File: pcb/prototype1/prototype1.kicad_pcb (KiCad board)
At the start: 2 copper layers, 73.4 x 73.4 mm, 87 parts, among them P5 USB_B, SW2 Button, SW3 Button, SW4 Button, SW5 Button, U1 STM32F401, U10 AT25_EEPROM, U11 LD1117S33CTR, U2 MP34DT01-M, U3 L3GD20HTR, U4 LIS331HH, U5 LIS331HH, U6 TPS61021, U7 TLC5926, U8 TLC5926, U9 TLC5926

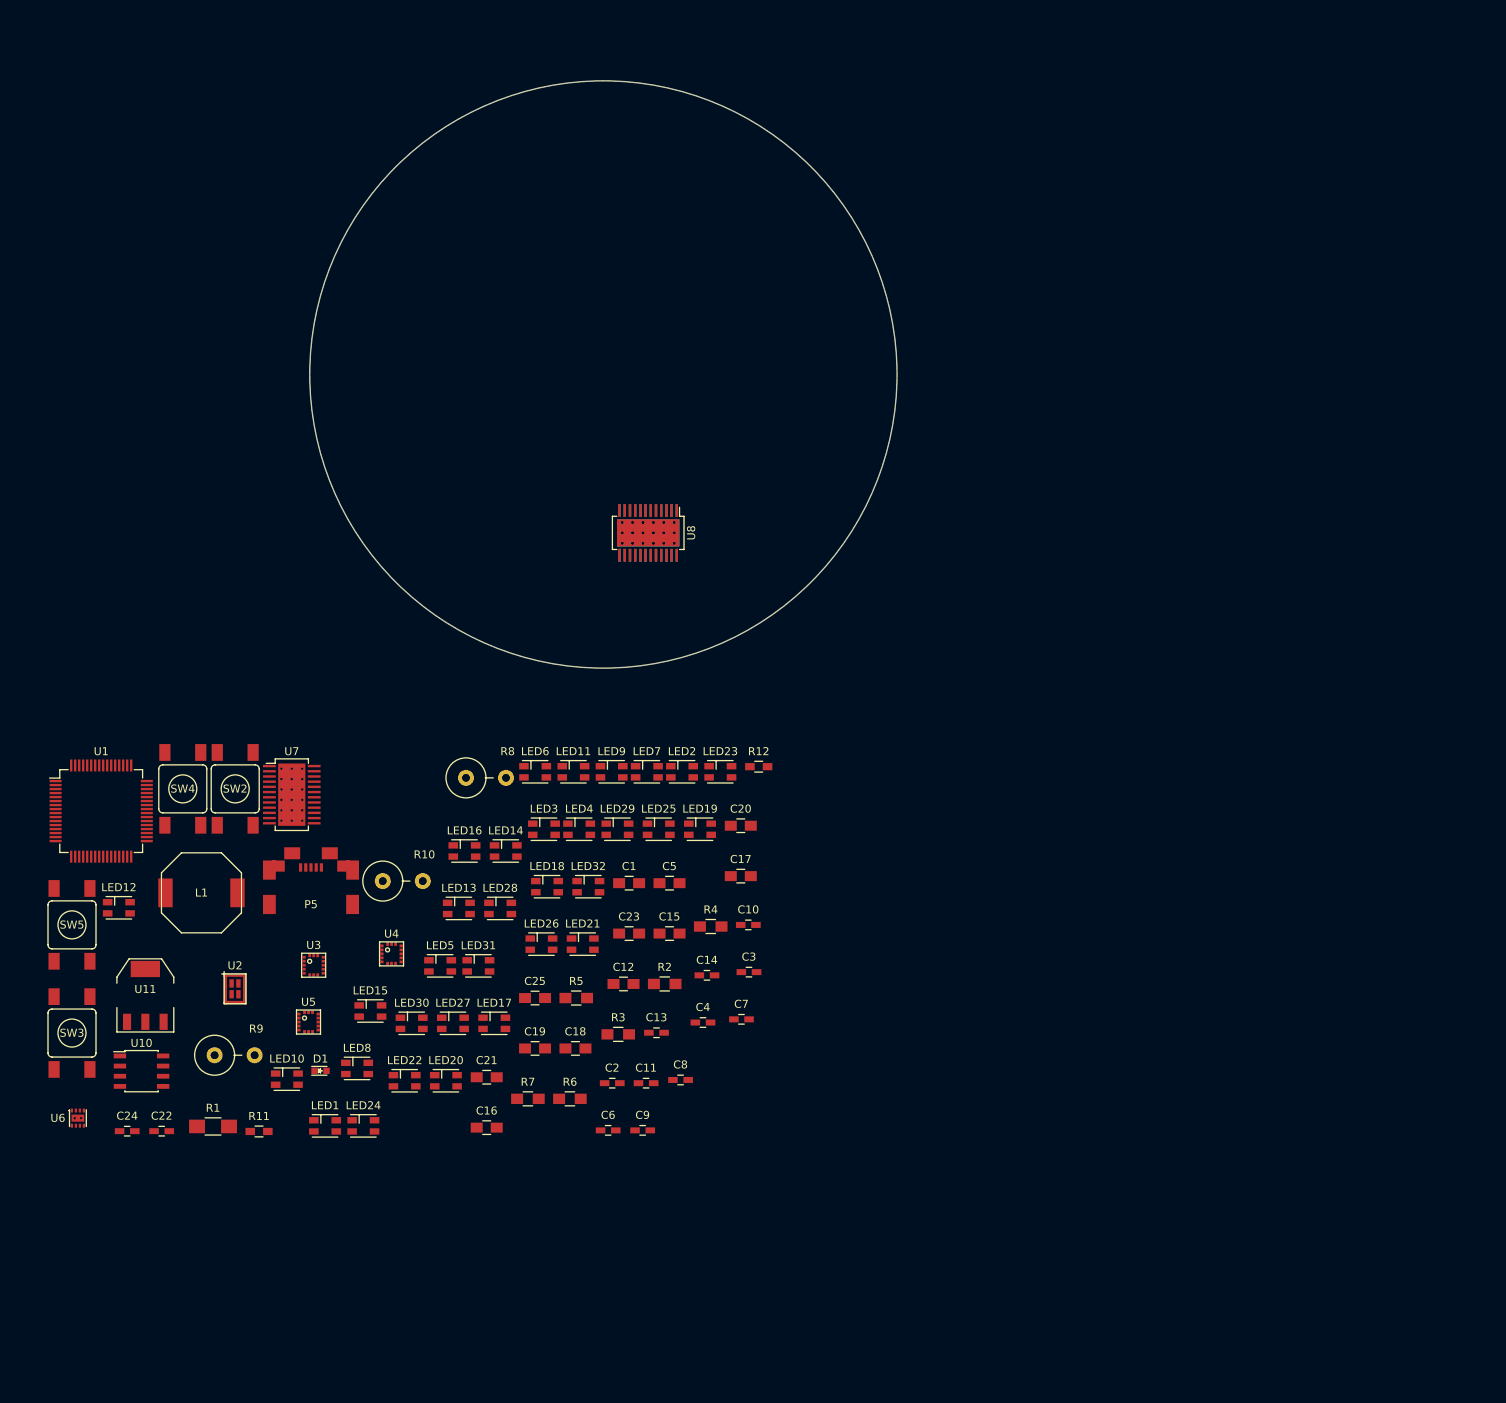
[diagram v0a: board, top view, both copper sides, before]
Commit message: Working on schematic
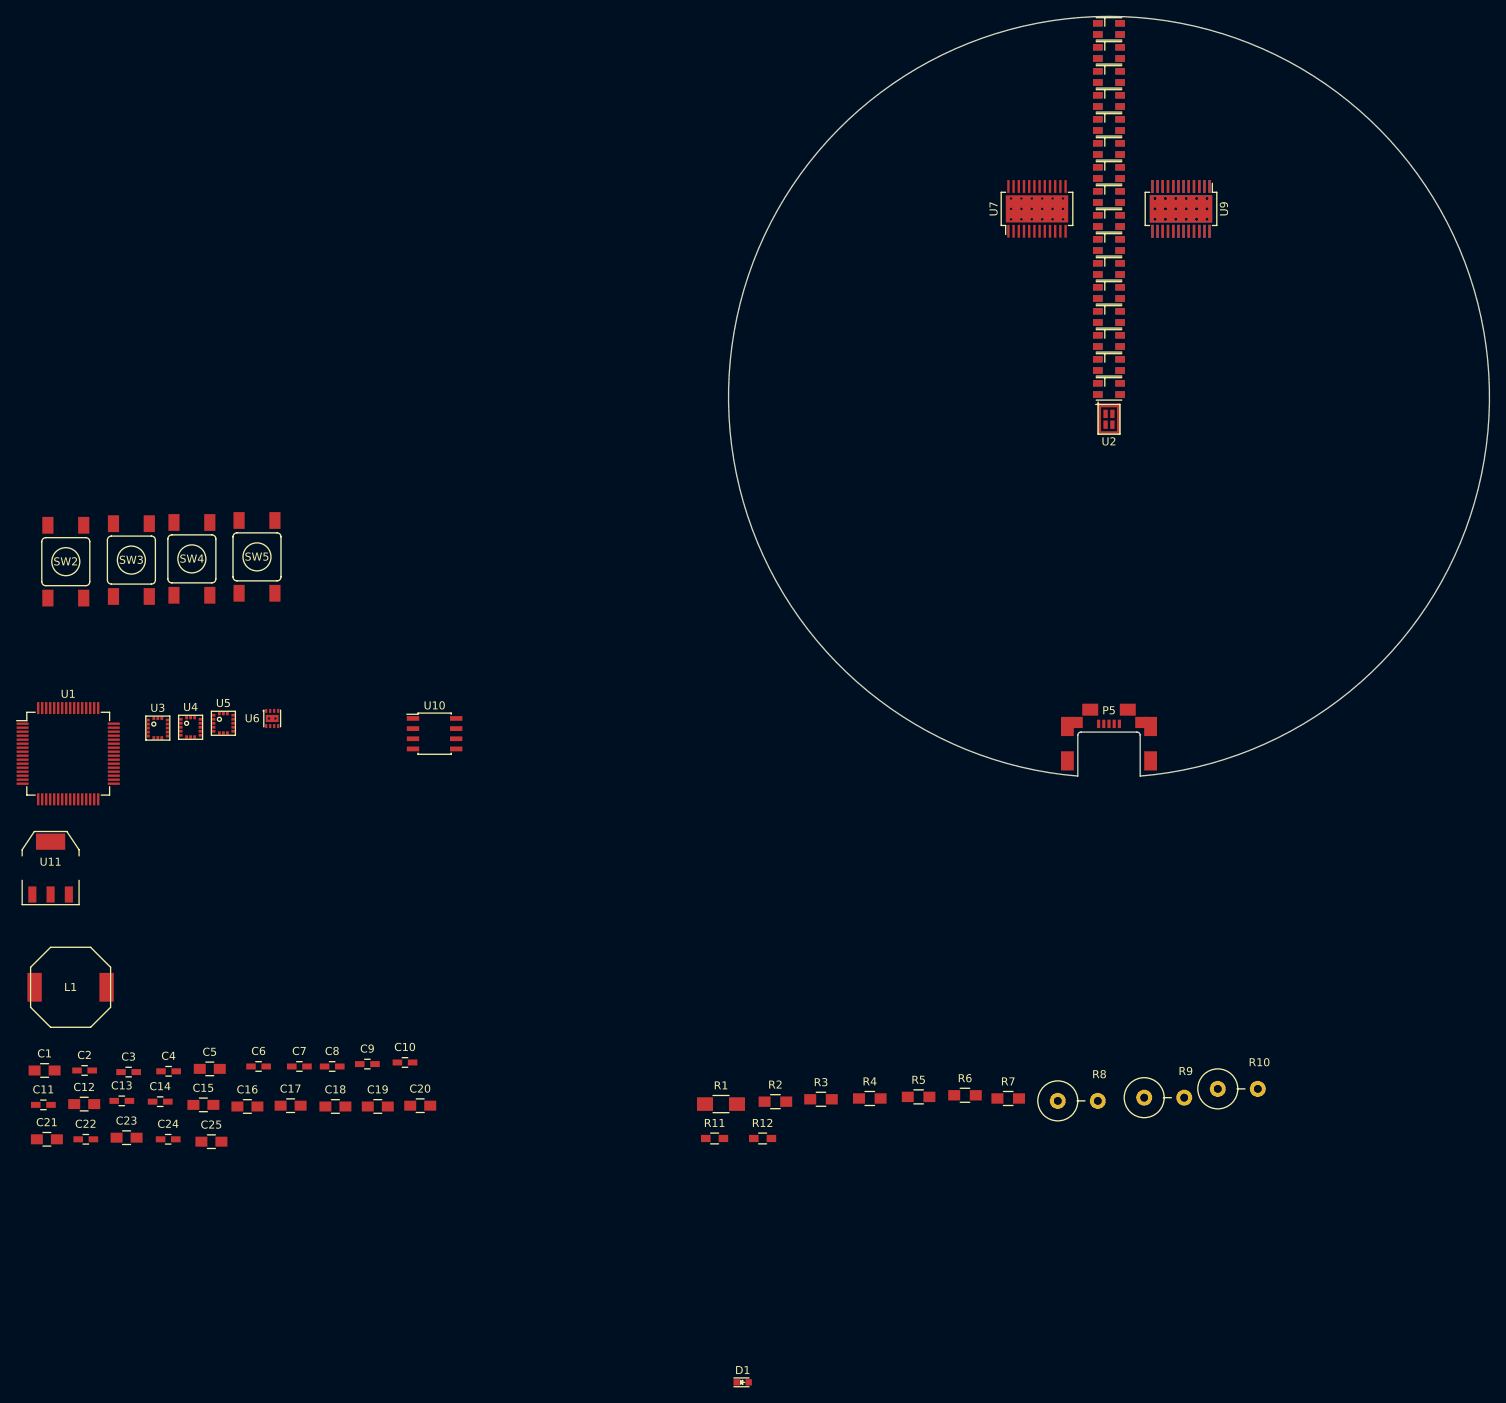
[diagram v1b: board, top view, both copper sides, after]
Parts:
- LED17, LED18, LED19, LED20, LED21, LED22, LED23, LED24, LED25, LED26, LED27, LED28, LED29, LED30, LED31, LED32, U8: moved to B.Cu
- U9: moved to F.Cu
- moved LED12 157.8 mm to (150.0, 66.0)
- moved LED10 153.0 mm to (150.0, 72.0)
- moved LED15 151.2 mm to (150.0, 57.0)
- moved LED30 146.9 mm to (150.0, 60.0)
- moved LED24 146.6 mm to (150.0, 78.0)
- moved LED8 141.6 mm to (150.0, 78.0)
- moved LED31 138.7 mm to (150.0, 57.0)
- moved LED27 136.6 mm to (150.0, 69.0)
- moved LED1 134.5 mm to (150.0, 99.0)
- moved LED22 134.4 mm to (150.0, 84.0)
- moved LED16 130.6 mm to (150.0, 54.0)
- moved U2 130.4 mm to (150.0, 102.8)
- moved LED13 129.6 mm to (150.0, 63.0)
- moved LED20 126.4 mm to (150.0, 90.0)
- moved LED32 125.4 mm to (150.0, 54.0)
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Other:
- board size 73.4 x 73.4 mm -> 95.1 x 95 mm
